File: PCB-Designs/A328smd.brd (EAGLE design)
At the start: 35.2 x 39.4 mm, 12 parts

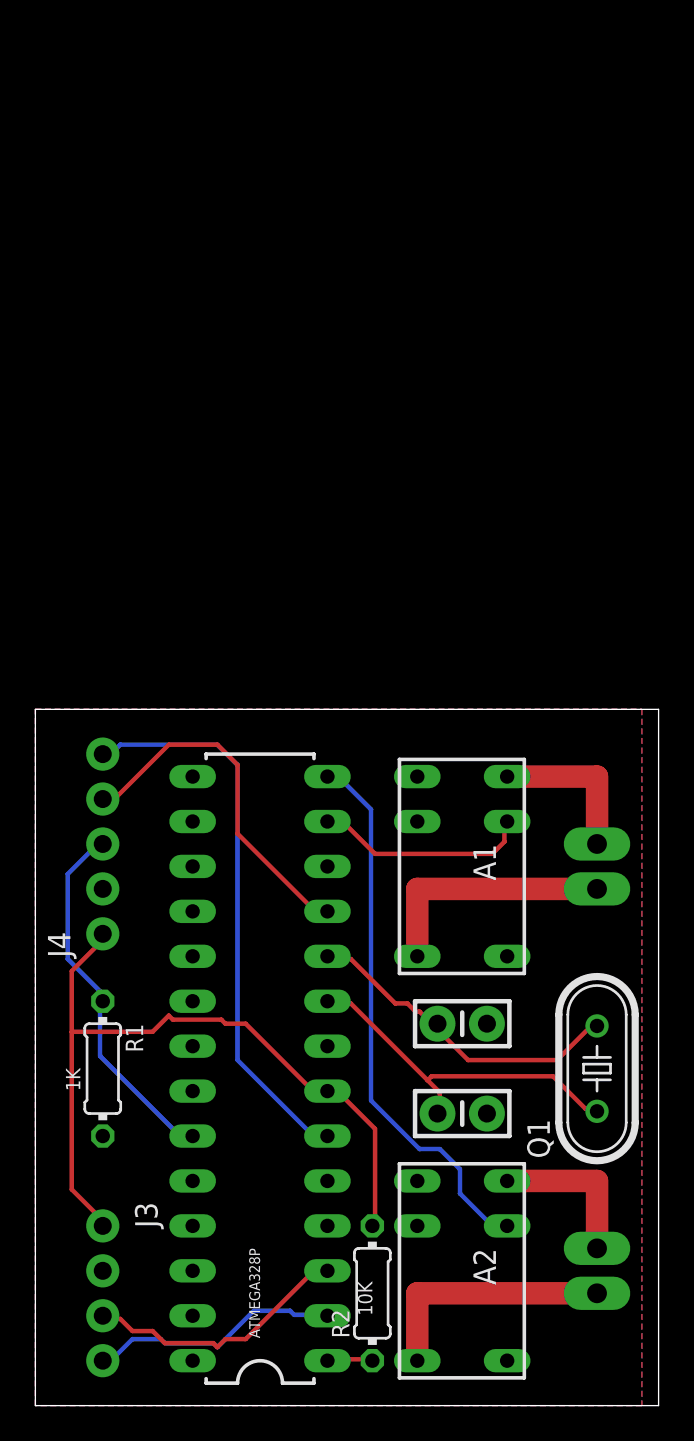
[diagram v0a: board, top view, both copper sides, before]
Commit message: Updating board files
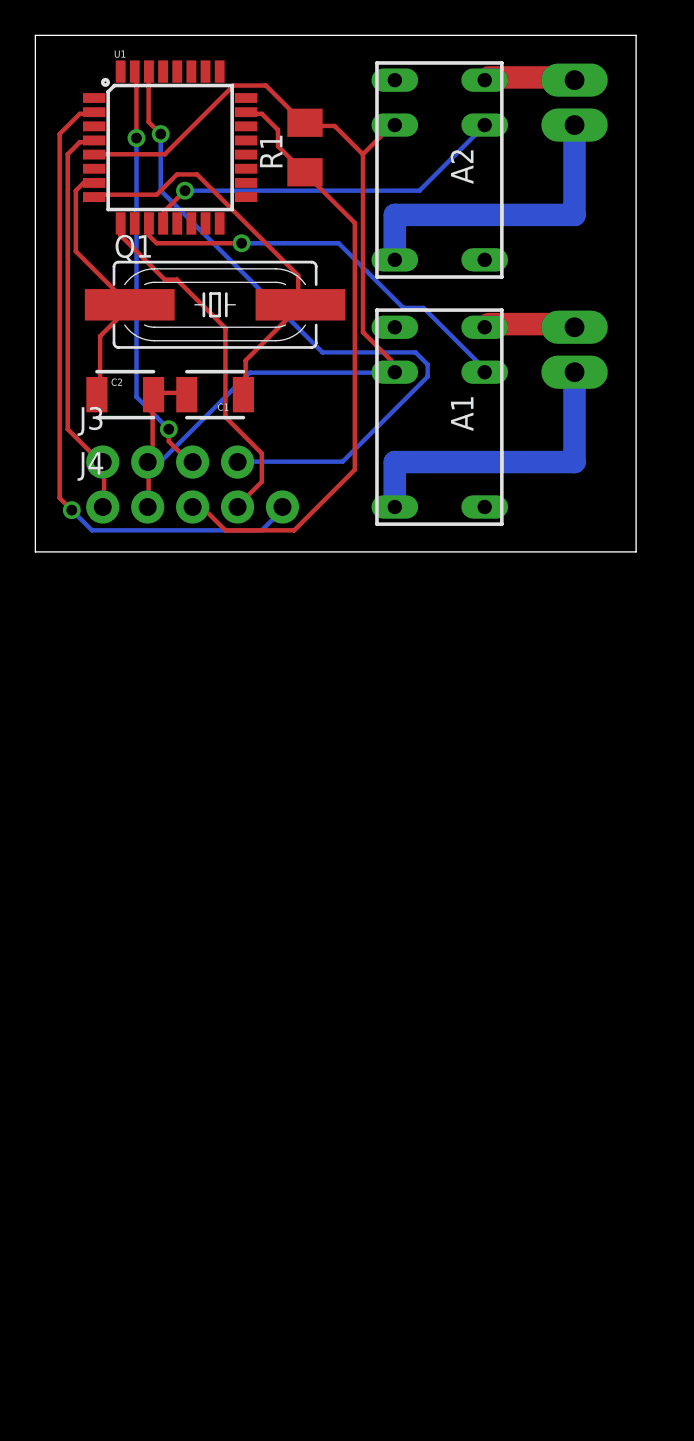
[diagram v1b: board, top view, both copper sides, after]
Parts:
- removed ATMEGA328P: ATMEGA328P_PDIP, SparkFun-DigitalIC:DIL28-3
- removed R2: 10K, resistor:0204/7
- added U1: ATMEGA328P_TQFP, SparkFun-DigitalIC:TQFP32-08
- C1, C2: device SparkFun-Capacitors:CAP-PTH-SMALL-KIT -> SparkFun-Capacitors:1210
- Q1: device crystal:HC49/S -> crystal:SM49
- R1: device resistor:0204/7 -> resistor:M1206
- moved J2 66.1 mm to (30.5, 73.7)
- moved A2 62.2 mm to (22.9, 71.1)
- moved R1 53.3 mm to (15.2, 72.4), turned to 90 degrees
- moved Q1 48.3 mm to (10.2, 63.5), turned to 0 degrees
- moved C2 44.9 mm to (5.08, 58.4)
- moved J3 43.2 mm to (3.81, 54.6), turned to 0 degrees
- moved C1 38.2 mm to (10.2, 58.4), turned to 180 degrees
- moved J1 29.2 mm to (30.5, 59.7)
- moved A1 25.4 mm to (22.9, 57.1)
- moved J4 24.1 mm to (3.81, 52.1), turned to 0 degrees
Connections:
- removed net RESET: ATMEGA328P.1, R2.1
- net +5V: now also U1.4; no longer ATMEGA328P.7, R2.2
- net A1: now also U1.11; no longer ATMEGA328P.13
- net A2: now also U1.12; no longer ATMEGA328P.14
- net ABTN: now also U1.23; no longer ATMEGA328P.23
- net GND: now also U1.5; no longer ATMEGA328P.22
- net GREEN: now also U1.9; no longer ATMEGA328P.11
- net OSC1: now also U1.7; no longer ATMEGA328P.9
- net OSC2: now also U1.8; no longer ATMEGA328P.10
- net RED: now also U1.2; no longer ATMEGA328P.6
- net RX: now also U1.30; no longer ATMEGA328P.2
- net TX: now also U1.31; no longer ATMEGA328P.3
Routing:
- net GND: track 0.00 -> 58.5 mm
- net RX: track 14.4 -> 39.6 mm, vias 0 -> 1
- net +5V: track 43.9 -> 22.7 mm
- net ABTN: track 21.0 -> 34.4 mm
- net A1: track 12.3 -> 23.0 mm, vias 0 -> 1
- net A2: track 31.1 -> 20.9 mm, vias 0 -> 1
- net TX: track 15.3 -> 23.5 mm, vias 0 -> 2
- net OSC1: track 20.2 -> 14.8 mm
- net RED: track 31.9 -> 37.0 mm, vias 0 -> 1
- net A2O: track 14.0 -> 17.8 mm
- net A1O: track 14.0 -> 17.8 mm
- net OSC2: track 18.9 -> 22.6 mm
- net A2I: track 8.89 -> 5.22 mm
- net A1I: track 8.89 -> 5.26 mm
- net RESET: track 2.59 -> 0.00 mm
- removed copper zone on layer 1, net GND
- removed copper zone on layer 16, net GND
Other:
- board size 35.2 x 39.4 mm -> 34 x 29.2 mm
- board text added: "ParrotStar V1.0"
- board text removed: "10K"
- board text removed: "1K"
- board text removed: "A"
- board text removed: "Aux1"
- board text removed: "Aux2"
- board text removed: "B"
- board text removed: "E"
- board text removed: "G"
- board text removed: "L"
- board text removed: "P"
- board text removed: "ParrotStar Beta 1"
- board text removed: "R"
- board text removed: "Y"
